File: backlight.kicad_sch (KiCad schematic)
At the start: 56 parts

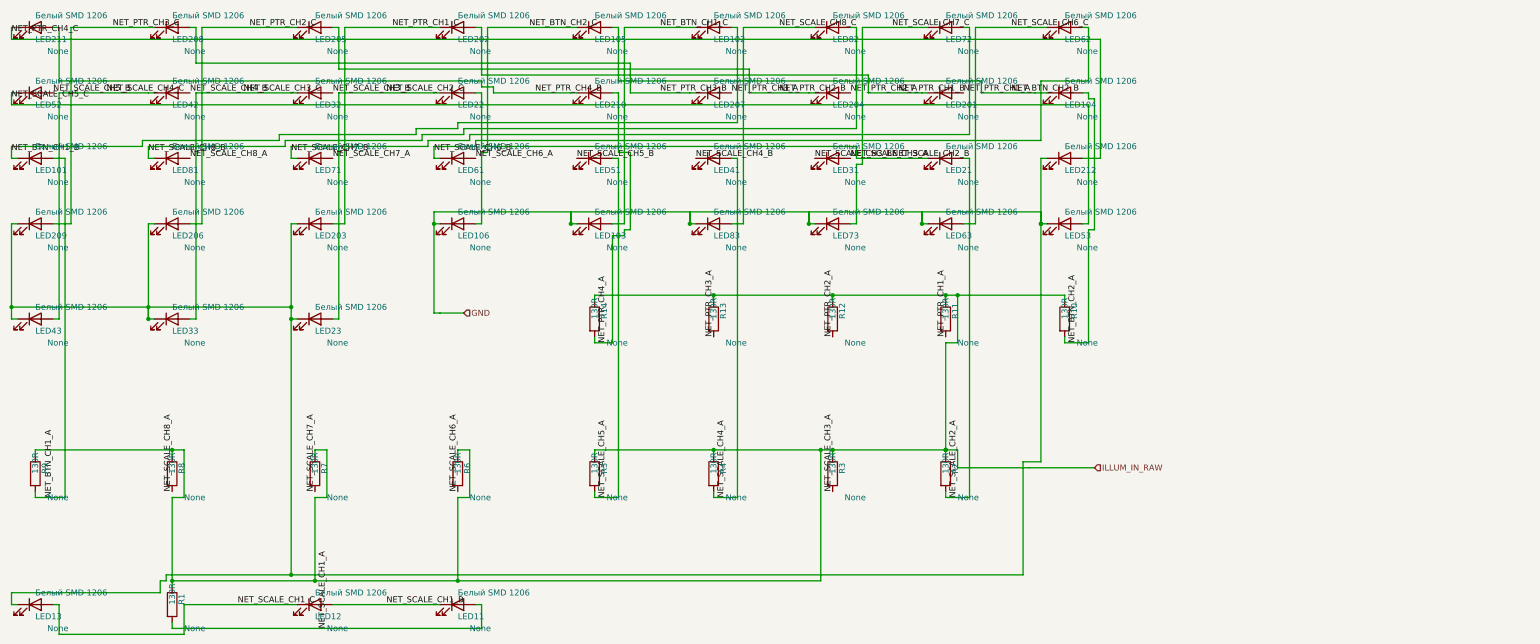
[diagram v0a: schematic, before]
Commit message: tests_fix
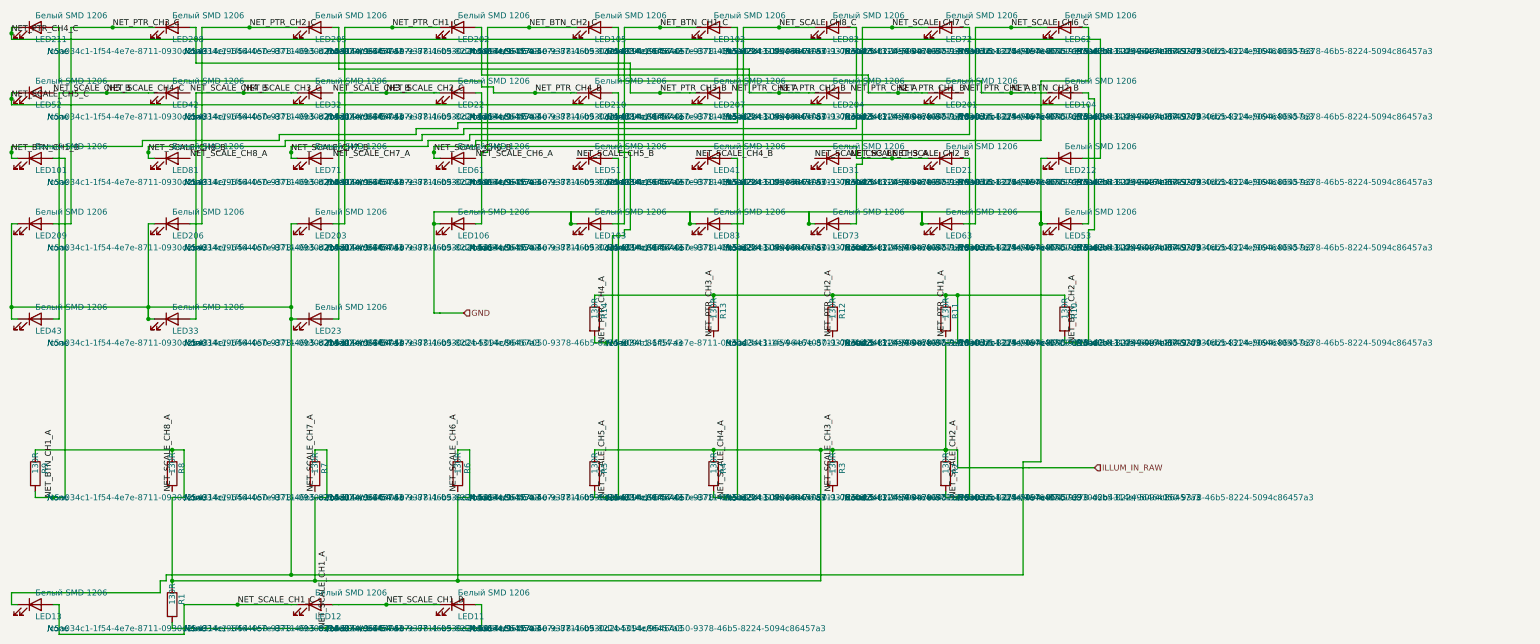
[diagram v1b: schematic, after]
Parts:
- LED101, LED102, LED103, LED104, LED105, LED106, LED11, LED12, LED13, LED201, LED202, LED203, LED204, LED205, LED206, LED207, LED208, LED209, LED21, LED210, LED211, LED212, LED22, LED23, LED31, LED32, LED33, LED41, LED42, LED43, LED51, LED52, LED53, LED61, LED62, LED63, LED71, LED72, LED73, LED81, LED82, LED83, R1, R10, R11, R12, R13, R14, R2, R3, R4, R5, R6, R7, R8, R9: hierarchy_path (none) -> /c5a034c1-1f54-4e7e-8711-0930d2b4314e/96464050-9378-46b5-82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
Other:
- title: (none) -> climate_control_niva_travel

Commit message: refactoring
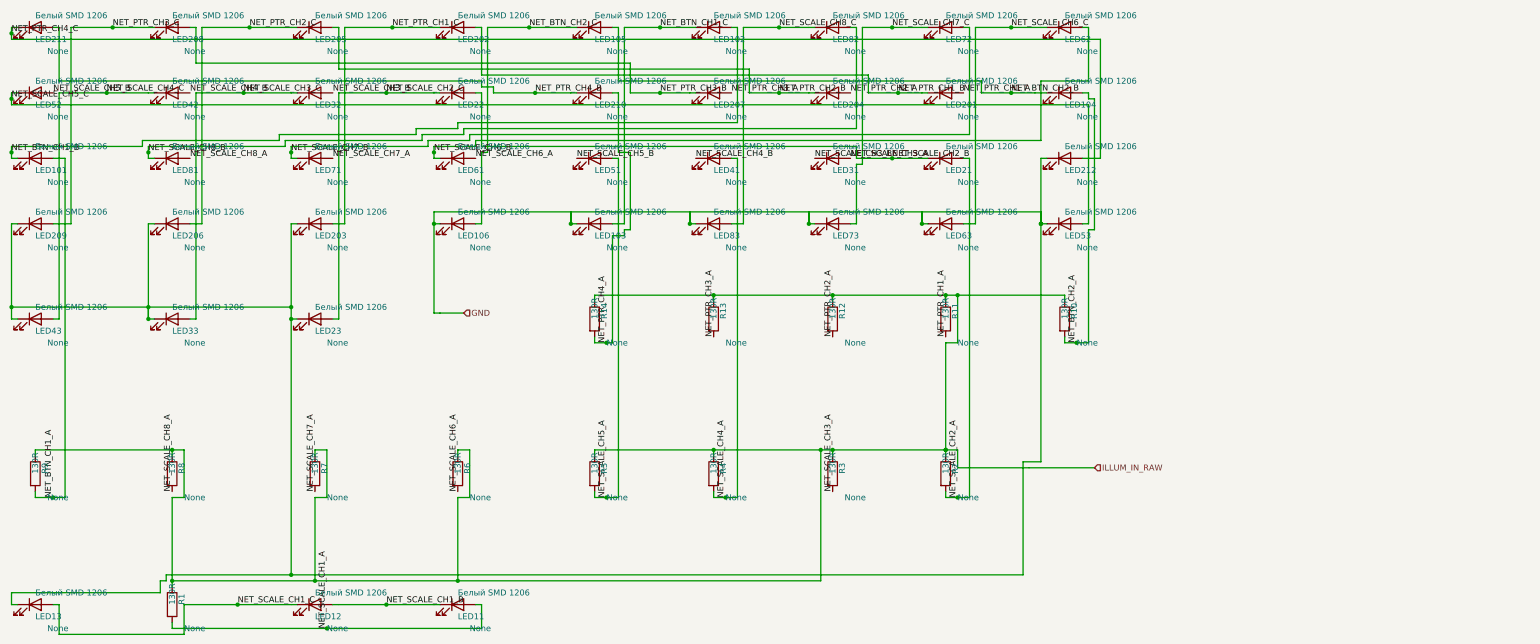
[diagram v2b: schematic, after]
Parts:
- LED101, LED102, LED103, LED104, LED105, LED106, LED11, LED12, LED13, LED201, LED202, LED203, LED204, LED205, LED206, LED207, LED208, LED209, LED21, LED210, LED211, LED212, LED22, LED23, LED31, LED32, LED33, LED41, LED42, LED43, LED51, LED52, LED53, LED61, LED62, LED63, LED71, LED72, LED73, LED81, LED82, LED83, R1, R10, R11, R12, R13, R14, R2, R3, R4, R5, R6, R7, R8, R9: hierarchy_path /c5a034c1-1f54-4e7e-8711-0930d2b4314e/96464050-9378-46b5-82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 -> (none)

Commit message: refactoring
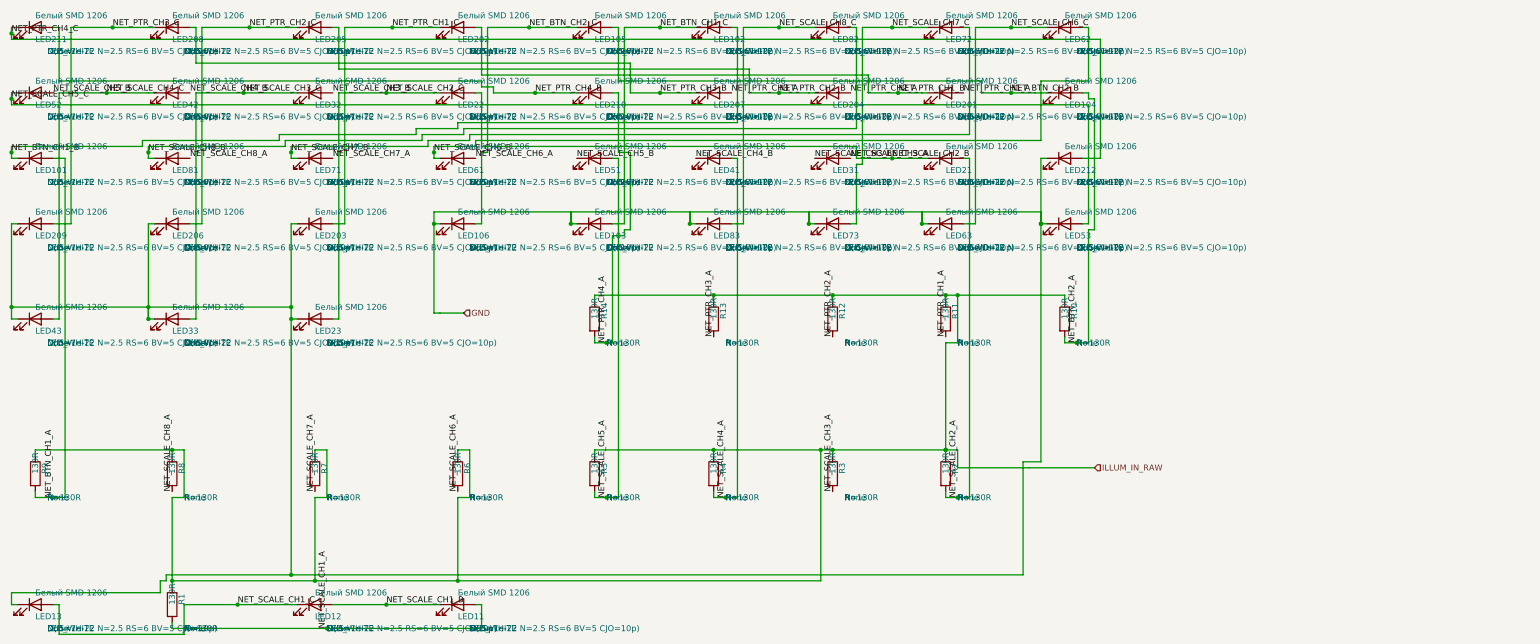
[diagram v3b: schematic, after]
